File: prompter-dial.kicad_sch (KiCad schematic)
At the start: 4 parts, among them SW1 JUMP_B, SW2 RUN, SW3 JUMP_F, U1 ATtiny85-20S

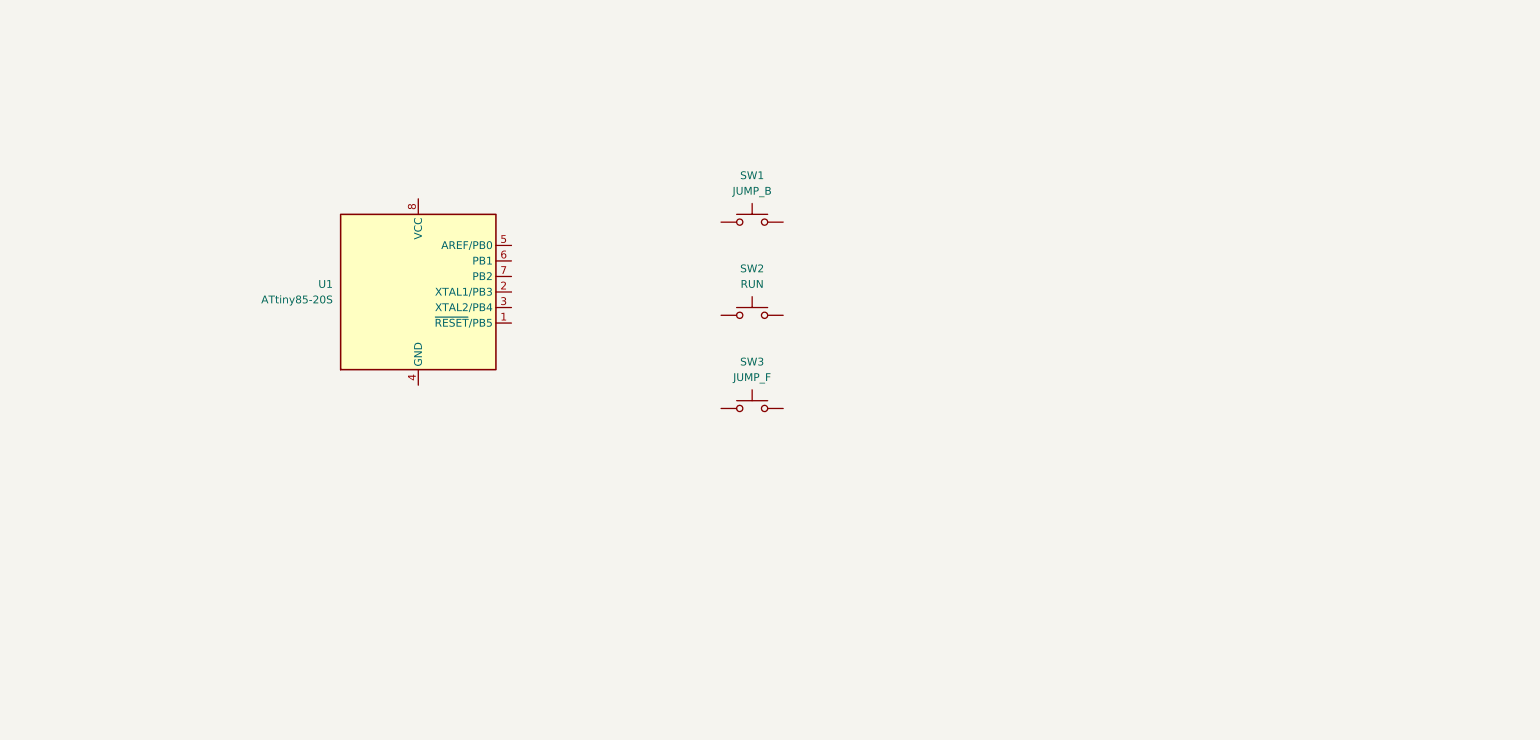
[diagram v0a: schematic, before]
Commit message: Create schematic
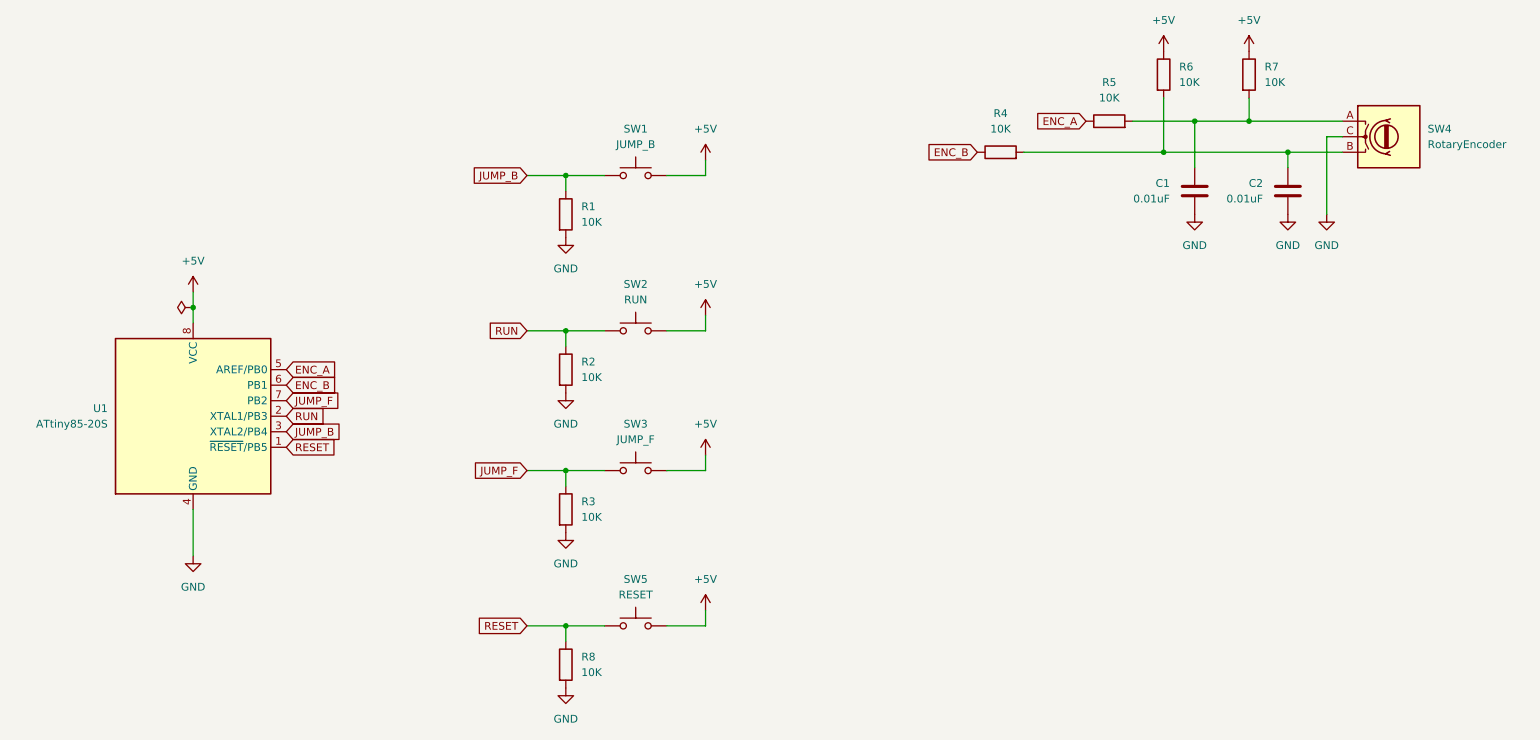
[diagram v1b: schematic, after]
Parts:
- added C1, C2: 0.01uF, symbol Device:C
- added R1, R2, R3, R4, R5, R6, R7, R8: 10K, symbol Device:R
- added SW4: RotaryEncoder, symbol Device:RotaryEncoder
- added SW5: RESET, Button_Switch_Keyboard:SW_Cherry_MX_1.00u_PCB, symbol Switch:SW_Push
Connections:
- net JUMP_F: now reaches SW3.1
- net JUMP_F: now also U1.7 (PB2), R3.1
- net +5V: now reaches SW3.2
- net +5V: now also SW1.2, SW2.2, U1.8 (VCC), R6.1, R7.1, SW5.2
- net JUMP_B: now reaches SW1.1
- net JUMP_B: now also U1.3 (XTAL2/PB4), R1.1
- net RUN: now reaches SW2.1
- net RUN: now also U1.2 (XTAL1/PB3), R2.1
- net RESET: now reaches U1.1 (~{RESET}/PB5)
- net RESET: now also R8.1, SW5.1
- net GND: now reaches U1.4 (GND)
- net GND: now also C1.2, C2.2, R1.2, R2.2, R3.2, R8.2, SW4.C
- net ENC_A: now reaches U1.5 (AREF/PB0)
- net ENC_A: now also R5.1
- net ENC_B: now reaches U1.6 (PB1)
- net ENC_B: now also R4.1
- new net: C1.1, R5.2, R7.2, SW4.A
- new net: C2.1, R4.2, R6.2, SW4.B
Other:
- moved on the sheet: SW3, U1
